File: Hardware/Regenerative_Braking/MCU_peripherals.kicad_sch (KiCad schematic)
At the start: 0 parts

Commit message: Added Battery side
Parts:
- added U1: NUCLEO-F446RE, NUCLEO-F446RE:MODULE_NUCLEO-F446RE, symbol Regen_braking:NUCLEO-F446RE
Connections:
- new net CN7_GND: U1.CN7_19 (CN7_GND), U1.CN7_20 (CN7_GND), U1.CN7_22 (CN7_GND), U1.CN7_8 (CN7_GND)

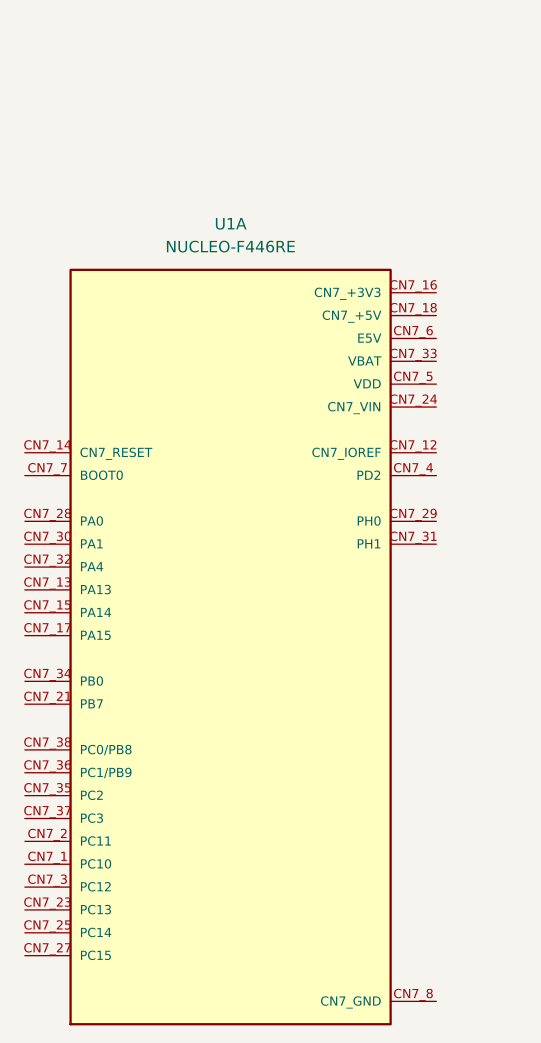
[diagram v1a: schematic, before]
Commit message: finished everything except mcu
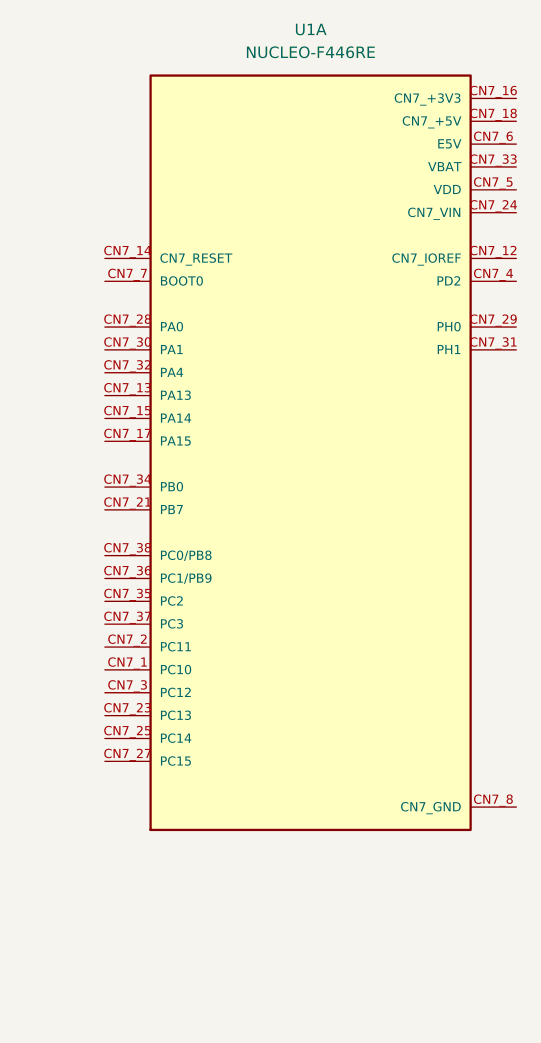
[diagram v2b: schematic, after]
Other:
- moved on the sheet: U1A
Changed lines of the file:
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@@
 	(symbol
 		(lib_id "Regen_braking:NUCLEO-F446RE")
-		(at 134.62 110.49 0)
+		(at 143.51 88.9 0)
 		(unit 1)
 		(body_style 1)
@@
 		(fields_autoplaced yes)
 		(property "Reference" "U1"
-			(at 134.62 64.77 0)
+			(at 143.51 43.18 0)
 			(show_name no)
 			(do_not_autoplace no)
@@
 		)
 		(property "Value" "NUCLEO-F446RE"
-			(at 134.62 67.31 0)
+			(at 143.51 45.72 0)
 			(show_name no)
 			(do_not_autoplace no)
@@
 		)
 		(property "Footprint" "NUCLEO-F446RE:MODULE_NUCLEO-F446RE"
-			(at 134.62 110.49 0)
+			(at 143.51 88.9 0)
 			(hide yes)
 			(show_name no)
@@
 		)
 		(property "Datasheet" ""
-			(at 134.62 110.49 0)
+			(at 143.51 88.9 0)
 			(hide yes)
 			(show_name no)
@@
 		)
 		(property "Description" "STM32F446RE, mbed-Enabled Development Nucleo-64 STM32F4 ARM® Cortex®-M4 MCU 32-Bit Embedded Evaluation Board"
-			(at 134.62 110.49 0)
+			(at 143.51 88.9 0)
 			(hide yes)
 			(show_name no)
@@
 		)
 		(property "MF" "STMicroelectronics"
-			(at 134.62 110.49 0)
+			(at 143.51 88.9 0)
 			(hide yes)
 			(show_name no)
@@
 		)
 		(property "MAXIMUM_PACKAGE_HEIGHT" ""
-			(at 134.62 110.49 0)
+			(at 143.51 88.9 0)
 			(hide yes)
 			(show_name no)
@@
 		)
 		(property "Package" "None"
-			(at 134.62 110.49 0)
+			(at 143.51 88.9 0)
 			(hide yes)
 			(show_name no)
@@
 		)
 		(property "Price" "None"
-			(at 134.62 110.49 0)
+			(at 143.51 88.9 0)
 			(hide yes)
 			(show_name no)
@@
 		)
 		(property "Check_prices" "https://www.snapeda.com/parts/NUCLEO-F446RE/STMicroelectronics/view-part/?ref=eda"
-			(at 134.62 110.49 0)
+			(at 143.51 88.9 0)
 			(hide yes)
 			(show_name no)
@@
 		)
 		(property "STANDARD" "Manufacturer Recommendations"
-			(at 134.62 110.49 0)
+			(at 143.51 88.9 0)
 			(hide yes)
 			(show_name no)
@@
 		)
 		(property "PARTREV" "13"
-			(at 134.62 110.49 0)
+			(at 143.51 88.9 0)
 			(hide yes)
 			(show_name no)
@@
 		)
 		(property "SnapEDA_Link" "https://www.snapeda.com/parts/NUCLEO-F446RE/STMicroelectronics/view-part/?ref=snap"
-			(at 134.62 110.49 0)
+			(at 143.51 88.9 0)
 			(hide yes)
 			(show_name no)
@@
 		)
 		(property "MP" "NUCLEO-F446RE"
-			(at 134.62 110.49 0)
+			(at 143.51 88.9 0)
 			(hide yes)
 			(show_name no)
@@
 		)
 		(property "Purchase-URL" "https://www.snapeda.com/api/url_track_click_mouser/?unipart_id=284290&manufacturer=STMicroelectronics&part_name=NUCLEO-F446RE&search_term=stm32 nucleo-64 development board with stm32f446re mcu"
-			(at 134.62 110.49 0)
+			(at 143.51 88.9 0)
 			(hide yes)
 			(show_name no)
@@
 		)
 		(property "Availability" "In Stock"
-			(at 134.62 110.49 0)
+			(at 143.51 88.9 0)
 			(hide yes)
 			(show_name no)
@@
 		)
 		(property "MANUFACTURER" "STMicroelectronics"
-			(at 134.62 110.49 0)
-			(hide yes)
-			(show_name no)
+			(at 143.51 88.9 0)
+			(hide yes)
+			(show_name no)

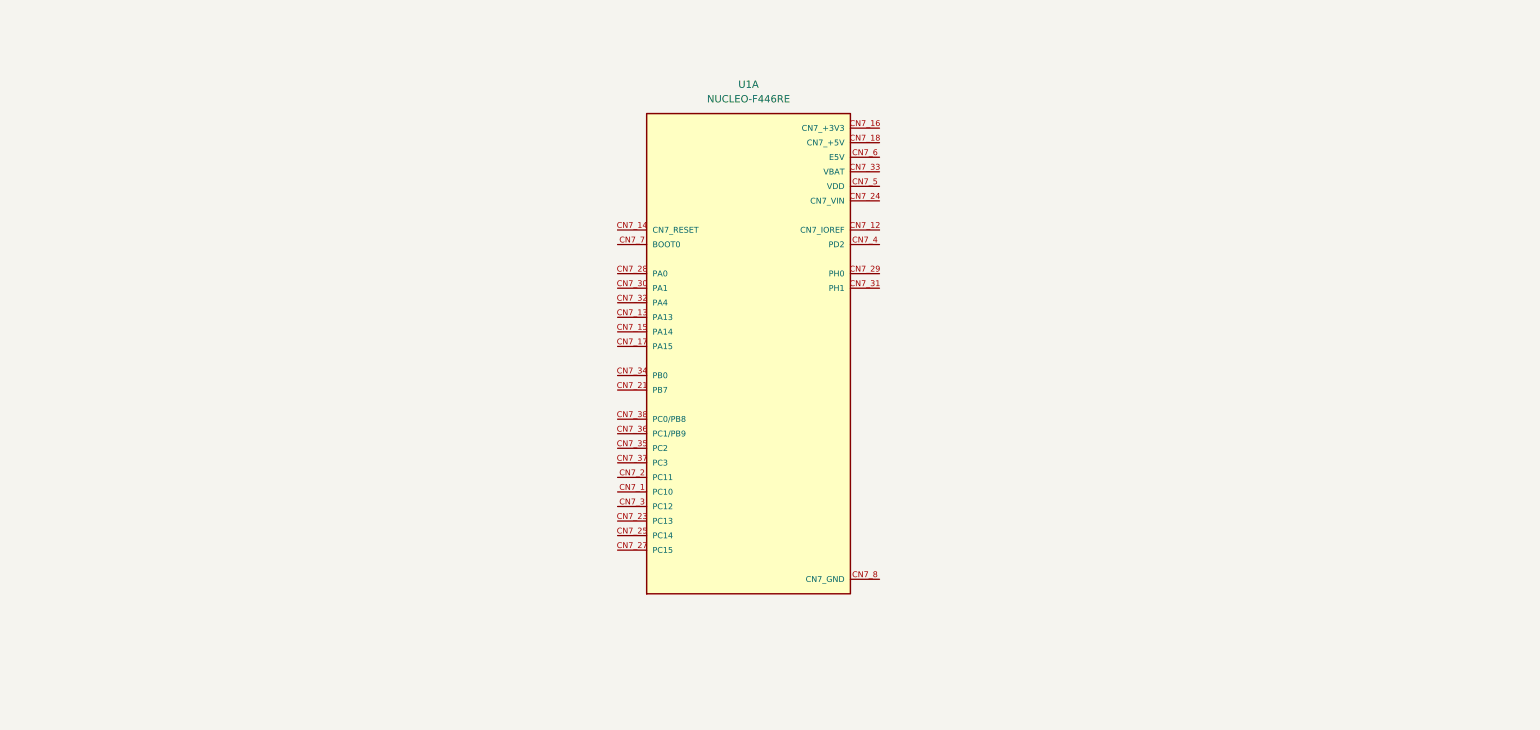
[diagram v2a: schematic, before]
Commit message: MCU CONNECTIONS
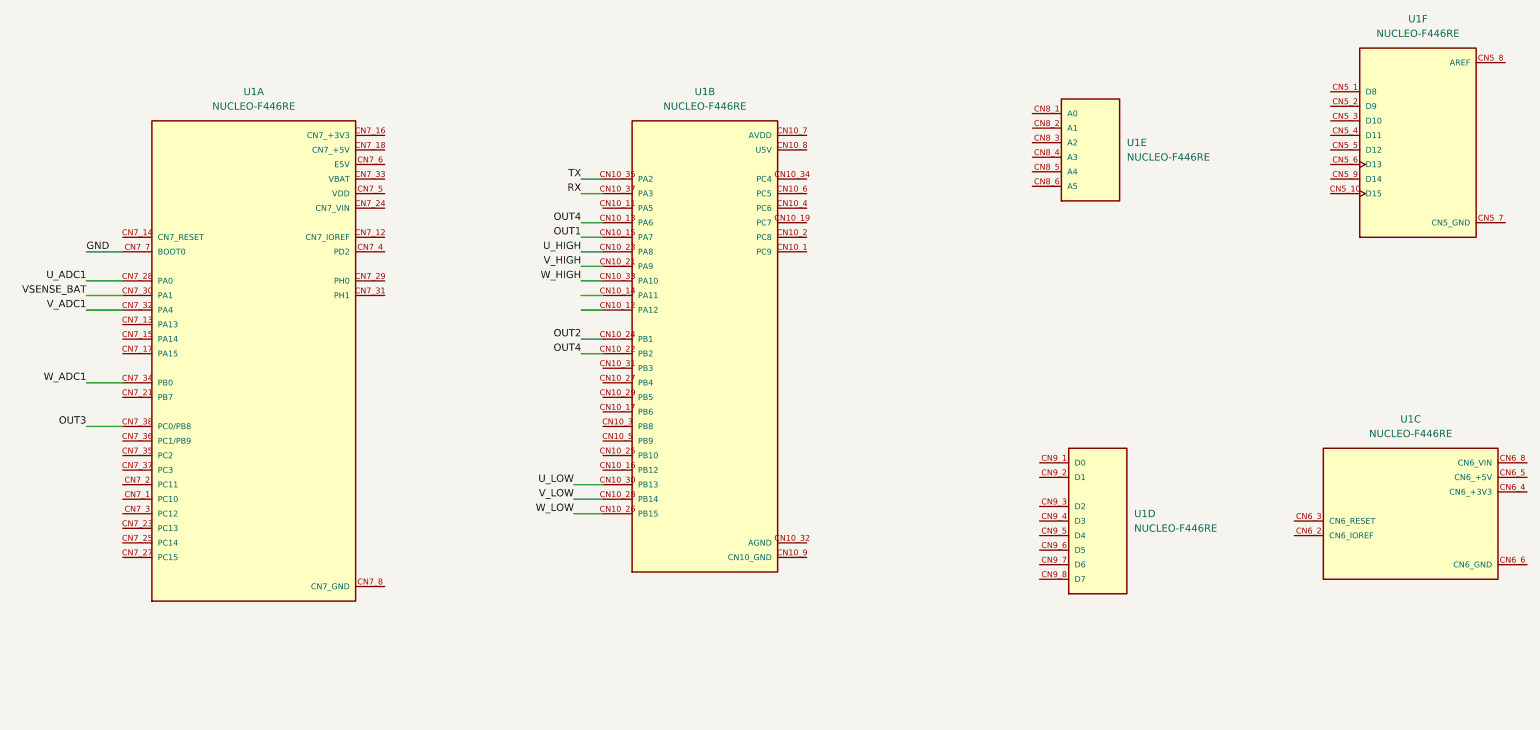
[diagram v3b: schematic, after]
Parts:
- added unit 6 of U1
- added unit 4 of U1
- added unit 5 of U1
- added unit 2 of U1
- added unit 3 of U1
- U1: footprint NUCLEO-F446RE:MODULE_NUCLEO-F446RE -> Regen_braking:MODULE_NUCLEO-F446RE
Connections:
- net U_ADC1: now reaches U1.CN7_28 (PA0)
- net VSENSE_BAT: now reaches U1.CN7_30 (PA1)
- net V_ADC1: now reaches U1.CN7_32 (PA4)
- net W_ADC1: now reaches U1.CN7_34 (PB0)
- net OUT3: now reaches U1.CN7_38 (PC0/PB8)
- net GND: now reaches U1.CN7_7 (BOOT0)
- new net CN10_GND: U1.CN10_20 (CN10_GND), U1.CN10_9 (CN10_GND)
- new net CN6_GND: U1.CN6_6 (CN6_GND), U1.CN6_7 (CN6_GND)
- new net OUT1: U1.CN10_15 (PA7)
- new net OUT2: U1.CN10_24 (PB1)
- new net OUT4: U1.CN10_13 (PA6), U1.CN10_22 (PB2)
- new net RX: U1.CN10_37 (PA3)
- new net TX: U1.CN10_35 (PA2)
- new net U_HIGH: U1.CN10_23 (PA8)
- new net U_LOW: U1.CN10_30 (PB13)
- new net V_HIGH: U1.CN10_21 (PA9)
- new net V_LOW: U1.CN10_28 (PB14)
- new net W_HIGH: U1.CN10_33 (PA10)
- new net W_LOW: U1.CN10_26 (PB15)
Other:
- moved on the sheet: U1A
